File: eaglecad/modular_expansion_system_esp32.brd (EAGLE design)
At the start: 90.2 x 100 mm, 34 parts, among them IC1 74LS30N, IC10 74LS244N, IC2 74LS04N, IC3 74LS04N, IC4 74LS00N, IC5 74LS04N, IC6 74LS74N, IC7 74LS00N, IC9 74S373N, J1 J1_ADDRESS_CON, J2 J2_DATA_AND_POWER_CON, J3 J3CONN, J3-WAIT WAIT, J4-INTERRUPTS INTERRUPTS, SW1 76SC04T, SW2 76SC04T, U1 ESP32-DEVKITC-32D

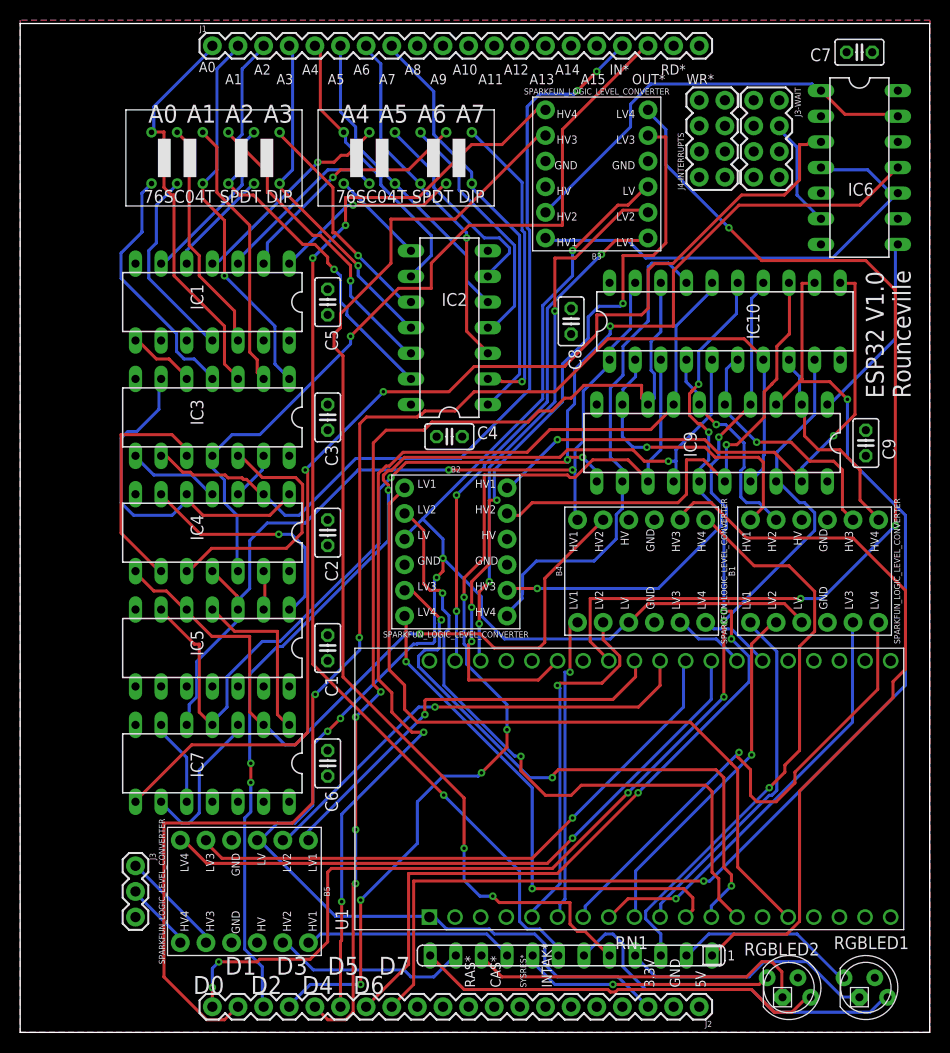
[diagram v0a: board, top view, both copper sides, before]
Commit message: updated esp32 board
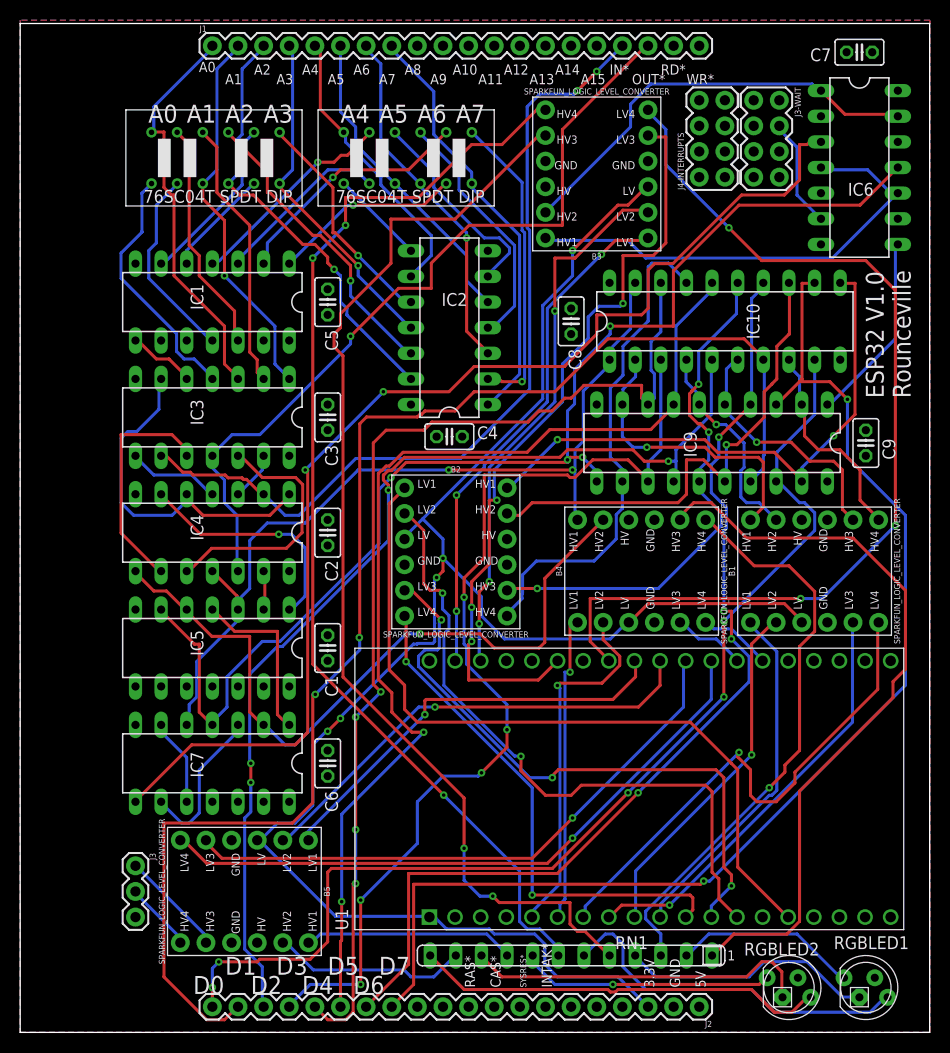
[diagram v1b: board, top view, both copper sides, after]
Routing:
- net D7: track 121.5 -> 120.5 mm
- net WIFI_OUT_LV_: track 37.0 -> 36.4 mm
- net D0: track 111.0 -> 110.4 mm
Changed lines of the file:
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@@
 <setting verticaltext="up"/>
 </settings>
-<grid distance="0.635" unitdist="mm" unit="mm" style="lines" multiple="1" display="no" altdistance="0.0635" altunitdist="mm" altunit="mm"/>
+<grid distance="0.3175" unitdist="mm" unit="mm" style="lines" multiple="1" display="no" altdistance="0.03175" altunitdist="mm" altunit="mm"/>
 <layers>
 <layer number="1" name="Top" color="4" fill="1" visible="yes" active="yes"/>
@@
 <wire x1="26.25" y1="51.25" x2="27.635" y2="51.25" width="0.3025" layer="16"/>
 <wire x1="24.25" y1="53.25" x2="26.25" y2="51.25" width="0.3025" layer="16"/>
-<wire x1="59.5" y1="97.75" x2="59.69" y2="97.79" width="0.3025" layer="16"/>
 <wire x1="24.25" y1="53.25" x2="24.13" y2="53.34" width="0.3025" layer="16"/>
 <wire x1="59.69" y1="97.79" x2="57.15" y2="95.25" width="0.3025" layer="16"/>
@@
 <contactref element="IC9" pad="18"/>
 <contactref element="IC10" pad="9"/>
-<wire x1="19.25" y1="2.75" x2="19.05" y2="2.54" width="0.3025" layer="16"/>
 <wire x1="75" y1="57.5" x2="75" y2="54.75" width="0.3025" layer="16"/>
 <wire x1="78.75" y1="61.25" x2="75" y2="57.5" width="0.3025" layer="16"/>
@@
 <wire x1="77.25" y1="52.5" x2="77.75" y2="52.5" width="0.3025" layer="16"/>
 <wire x1="75" y1="54.75" x2="77.25" y2="52.5" width="0.3025" layer="16"/>
-<wire x1="19.25" y1="2.75" x2="19.05" y2="2.54" width="0.3025" layer="1"/>
 <wire x1="75" y1="54.75" x2="74.93" y2="54.61" width="0.3025" layer="16"/>
 <via x="60.25" y="23.75" extent="1-16" drill="0.35"/>
@@
 <contactref element="IC9" pad="14"/>
 <contactref element="IC10" pad="5"/>
-<wire x1="24.25" y1="2.75" x2="24.13" y2="2.54" width="0.3025" layer="1"/>
 <wire x1="65" y1="57.75" x2="65" y2="56.615" width="0.3025" layer="16"/>
 <wire x1="65" y1="56.615" x2="65" y2="54.75" width="0.3025" layer="16"/>
@@
 <contactref element="IC9" pad="13"/>
 <contactref element="IC10" pad="3"/>
-<wire x1="26.5" y1="2.75" x2="26.67" y2="2.54" width="0.3025" layer="1"/>
 <wire x1="62.25" y1="56.5" x2="62.25" y2="54.75" width="0.3025" layer="16"/>
 <wire x1="63.5" y1="57.75" x2="62.25" y2="56.5" width="0.3025" layer="16"/>
@@
 <contactref element="IC9" pad="7"/>
 <contactref element="IC10" pad="16"/>
-<wire x1="31.75" y1="2.75" x2="31.75" y2="2.54" width="0.3025" layer="16"/>
 <wire x1="65" y1="70" x2="65" y2="62.25" width="0.3025" layer="16"/>
 <wire x1="68.5" y1="73.5" x2="65" y2="70" width="0.3025" layer="16"/>
@@
 <wire x1="65" y1="62.25" x2="64.77" y2="62.23" width="0.3025" layer="16"/>
 <wire x1="68.5" y1="74.25" x2="68.58" y2="74.295" width="0.3025" layer="16"/>
-<wire x1="31.75" y1="9" x2="31.75" y2="2.54" width="0.3025" layer="1"/>
-<wire x1="31.865" y1="9.115" x2="31.75" y2="9" width="0.3025" layer="1"/>
+<wire x1="31.75" y1="9" x2="31.865" y2="9.115" width="0.3025" layer="1"/>
 <wire x1="31.865" y1="12.96" x2="31.865" y2="9.115" width="0.3025" layer="1"/>
 <wire x1="31.865" y1="21.615" x2="31.865" y2="12.96" width="0.3025" layer="16"/>
@@
 <wire x1="35.5" y1="55.38833125" x2="35.5" y2="35" width="0.3025" layer="1"/>
 <wire x1="36.27913125" y1="56.13675" x2="35.84228125" y2="55.6999" width="0.3025" layer="1"/>
+<wire x1="31.75" y1="2.54" x2="31.75" y2="9" width="0.3025" layer="1"/>
 </signal>
 <signal name="D6">
@@
 <contactref element="IC9" pad="4"/>
 <contactref element="IC10" pad="14"/>
-<wire x1="34.5" y1="2.75" x2="34.29" y2="2.54" width="0.3025" layer="16"/>
 <wire x1="72.5" y1="72.75" x2="72.5" y2="62.25" width="0.3025" layer="16"/>
 <wire x1="73.5" y1="73.75" x2="72.5" y2="72.75" width="0.3025" layer="16"/>
@@
 <wire x1="72.5" y1="62.25" x2="72.39" y2="62.23" width="0.3025" layer="16"/>
 <wire x1="73.5" y1="74.25" x2="73.66" y2="74.295" width="0.3025" layer="16"/>
-<wire x1="38.5" y1="6.75" x2="34.29" y2="2.54" width="0.3025" layer="1"/>
-<wire x1="38.5" y1="15.75" x2="38.5" y2="6.75" width="0.3025" layer="1"/>
+<wire x1="38.5" y1="6.75" x2="38.5" y2="15.75" width="0.3025" layer="1"/>
 <wire x1="53.25" y1="15.75" x2="38.5" y2="15.75" width="0.3025" layer="1"/>
 <wire x1="61.25" y1="23.75" x2="53.25" y2="15.75" width="0.3025" layer="1"/>
@@
 <via x="69.75" y="41.75" extent="1-16" drill="0.35"/>
 <via x="69.25" y="59" extent="1-16" drill="0.35"/>
+<wire x1="34.29" y1="2.54" x2="38.5" y2="6.75" width="0.3025" layer="1"/>
 </signal>
 <signal name="D7">
@@
 <contactref element="IC9" pad="3"/>
 <contactref element="IC10" pad="12"/>
-<wire x1="37" y1="2.75" x2="37.5" y2="2.75" width="0.3025" layer="16"/>
-<wire x1="37" y1="2.75" x2="36.83" y2="2.54" width="0.3025" layer="16"/>
 <wire x1="77.5" y1="64.75" x2="77.25" y2="64.5" width="0.3025" layer="1"/>
 <wire x1="77.25" y1="64.5" x2="75" y2="62.25" width="0.3025" layer="1"/>
@@
 <wire x1="75" y1="62.25" x2="74.93" y2="62.23" width="0.3025" layer="1"/>
 <wire x1="78.5" y1="74.25" x2="78.74" y2="74.295" width="0.3025" layer="1"/>
-<wire x1="39" y1="4.75" x2="37" y2="2.75" width="0.3025" layer="1"/>
-<wire x1="39" y1="15" x2="39" y2="4.75" width="0.3025" layer="1"/>
-<wire x1="67.75" y1="15" x2="39" y2="15" width="0.3025" layer="1"/>
+<wire x1="37" y1="2.75" x2="39" y2="4.75" width="0.3025" layer="1"/>
+<wire x1="39" y1="14.6825" x2="39" y2="4.75" width="0.3025" layer="1"/>
+<wire x1="67.75" y1="15" x2="67.4325" y2="14.6825" width="0.3025" layer="1"/>
+<wire x1="67.4325" y1="14.6825" x2="39" y2="14.6825" width="0.3025" layer="1"/>
 <wire x1="87.75" y1="51.25" x2="82" y2="57" width="0.3025" layer="16"/>
 <wire x1="82" y1="62.75" x2="82" y2="57" width="0.3025" layer="16"/>
 <wire x1="80.25" y1="64.5" x2="82" y2="62.75" width="0.3025" layer="1"/>
 <wire x1="77.25" y1="64.5" x2="80.25" y2="64.5" width="0.3025" layer="1"/>
-<wire x1="37" y1="2.75" x2="36.83" y2="2.54" width="0.3025" layer="1"/>
 <via x="67.75" y="15" extent="1-16" drill="0.35"/>
 <via x="82" y="62.75" extent="1-16" drill="0.35"/>
@@
 <wire x1="68.34" y1="15" x2="87.75" y2="34.41" width="0.3025" layer="16"/>
 <wire x1="87.75" y1="34.41" x2="87.75" y2="51.25" width="0.3025" layer="16"/>
+<wire x1="36.83" y1="2.54" x2="37" y2="2.71" width="0.3025" layer="1"/>
+<wire x1="37" y1="2.71" x2="37" y2="2.75" width="0.3025" layer="1"/>
 </signal>
 <signal name="RAS*">
@@
 <wire x1="10" y1="52.5" x2="11.25" y2="51.25" width="0.3025" layer="16"/>
 <wire x1="13.75" y1="64.75" x2="13.97" y2="64.77" width="0.3025" layer="16"/>
-<wire x1="16.5" y1="53.5" x2="16.51" y2="53.34" width="0.3025" layer="16"/>
 <wire x1="10.665" y1="59.56" x2="11.56" y2="59.56" width="0.3025" layer="16"/>
 <wire x1="10" y1="52.5" x2="10" y2="58.895" width="0.3025" layer="16"/>
@@
 <contactref element="U1" pad="8"/>
 <contactref element="B1" pad="LV3"/>
-<wire x1="60.25" y1="13.25" x2="58.5" y2="11.5" width="0.3025" layer="1"/>
-<wire x1="65" y1="13.25" x2="60.25" y2="13.25" width="0.3025" layer="1"/>
-<wire x1="82.5" y1="30.75" x2="65" y2="13.25" width="0.3025" layer="16"/>
+<wire x1="59.615" y1="12.615" x2="58.5" y2="11.5" width="0.3025" layer="1"/>
+<wire x1="64.365" y1="12.615" x2="59.615" y2="12.615" width="0.3025" layer="1"/>
+<wire x1="82.5" y1="30.75" x2="64.365" y2="12.615" width="0.3025" layer="16"/>
 <wire x1="82.5" y1="40.5" x2="82.5" y2="30.75" width="0.3025" layer="16"/>
 <wire x1="58.5" y1="11.5" x2="58.345" y2="11.43" width="0.3025" layer="1"/>
 <wire x1="82.5" y1="40.5" x2="82.55" y2="40.64" width="0.3025" layer="16"/>
-<via x="65" y="13.25" extent="1-16" drill="0.35"/>
+<via x="64.365" y="12.615" extent="1-16" drill="0.35"/>
 </signal>
 <signal name="D5_LV">
@@
 <contactref element="U1" pad="11"/>
 <contactref element="B2" pad="LV4"/>
-<wire x1="50.75" y1="14.25" x2="65.75" y2="14.25" width="0.3025" layer="1"/>
-<wire x1="50.75" y1="24.25" x2="50.75" y2="14.25" width="0.3025" layer="16"/>
+<wire x1="66.395" y1="13.615" x2="50.75" y2="13.615" width="0.3025" layer="1"/>
+<wire x1="50.75" y1="24.25" x2="50.75" y2="13.615" width="0.3025" layer="16"/>
 <wire x1="38.25" y1="36.75" x2="50.75" y2="24.25" width="0.3025" layer="16"/>
 <wire x1="38.25" y1="41.25" x2="38.25" y2="36.75" width="0.3025" layer="1"/>
 <wire x1="38.25" y1="41.25" x2="38.1" y2="41.275" width="0.3025" layer="1"/>
-<via x="50.75" y="14.25" extent="1-16" drill="0.35"/>
+<via x="50.75" y="13.615" extent="1-16" drill="0.35"/>
 <via x="38.25" y="36.75" extent="1-16" drill="0.35"/>
-<wire x1="65.75" y1="14.25" x2="65.76" y2="14.25" width="0.3025" layer="1"/>
 <wire x1="66.675" y1="13.335" x2="66.675" y2="12.14" width="0.3025" layer="1"/>
 <wire x1="66.675" y1="12.14" x2="65.965" y2="11.43" width="0.3025" layer="1"/>
-<wire x1="65.76" y1="14.25" x2="66.675" y2="13.335" width="0.3025" layer="1"/>
+<wire x1="66.395" y1="13.615" x2="66.675" y2="13.335" width="0.3025" layer="1"/>
 </signal>
 <signal name="D2_LV">
@@
 <wire x1="50.5" y1="11.5" x2="50.725" y2="11.43" width="0.3025" layer="16"/>
 <via x="53.25" y="34.385" extent="1-16" drill="0.35"/>
-<wire x1="57.785" y1="40.64" x2="57.785" y2="40.005" width="0.3025" layer="1"/>
 <wire x1="59.42865" y1="37.27886875" x2="59.42865" y2="36.38113125" width="0.3025" layer="1"/>
 <wire x1="59.42865" y1="36.38113125" x2="57.66251875" y2="34.615" width="0.3025" layer="1"/>
 <wire x1="57.66251875" y1="34.615" x2="53.48" y2="34.615" width="0.3025" layer="1"/>
-<wire x1="57.785" y1="40.64" x2="57.785" y2="38.92251875" width="0.3025" layer="1"/>
-<wire x1="57.785" y1="38.92251875" x2="59.42865" y2="37.27886875" width="0.3025" layer="1"/>
+<wire x1="59.42865" y1="37.27886875" x2="57.785" y2="38.92251875" width="0.3025" layer="1"/>
+<wire x1="57.785" y1="38.92251875" x2="57.785" y2="40.64" width="0.3025" layer="1"/>
 </signal>
 <signal name="WIFI_IN">
